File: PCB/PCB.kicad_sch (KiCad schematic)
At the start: 45 parts, among them J2 USB_C_Receptacle_USB2.0_16P, J4 Conn_01x15_Pin, J5 Conn_01x15_Pin, SW1 SW_Push, SW2 SW_Push, U2 ESP32-S3FN8, U3 TPS63900DSKR, Y1 40MHz

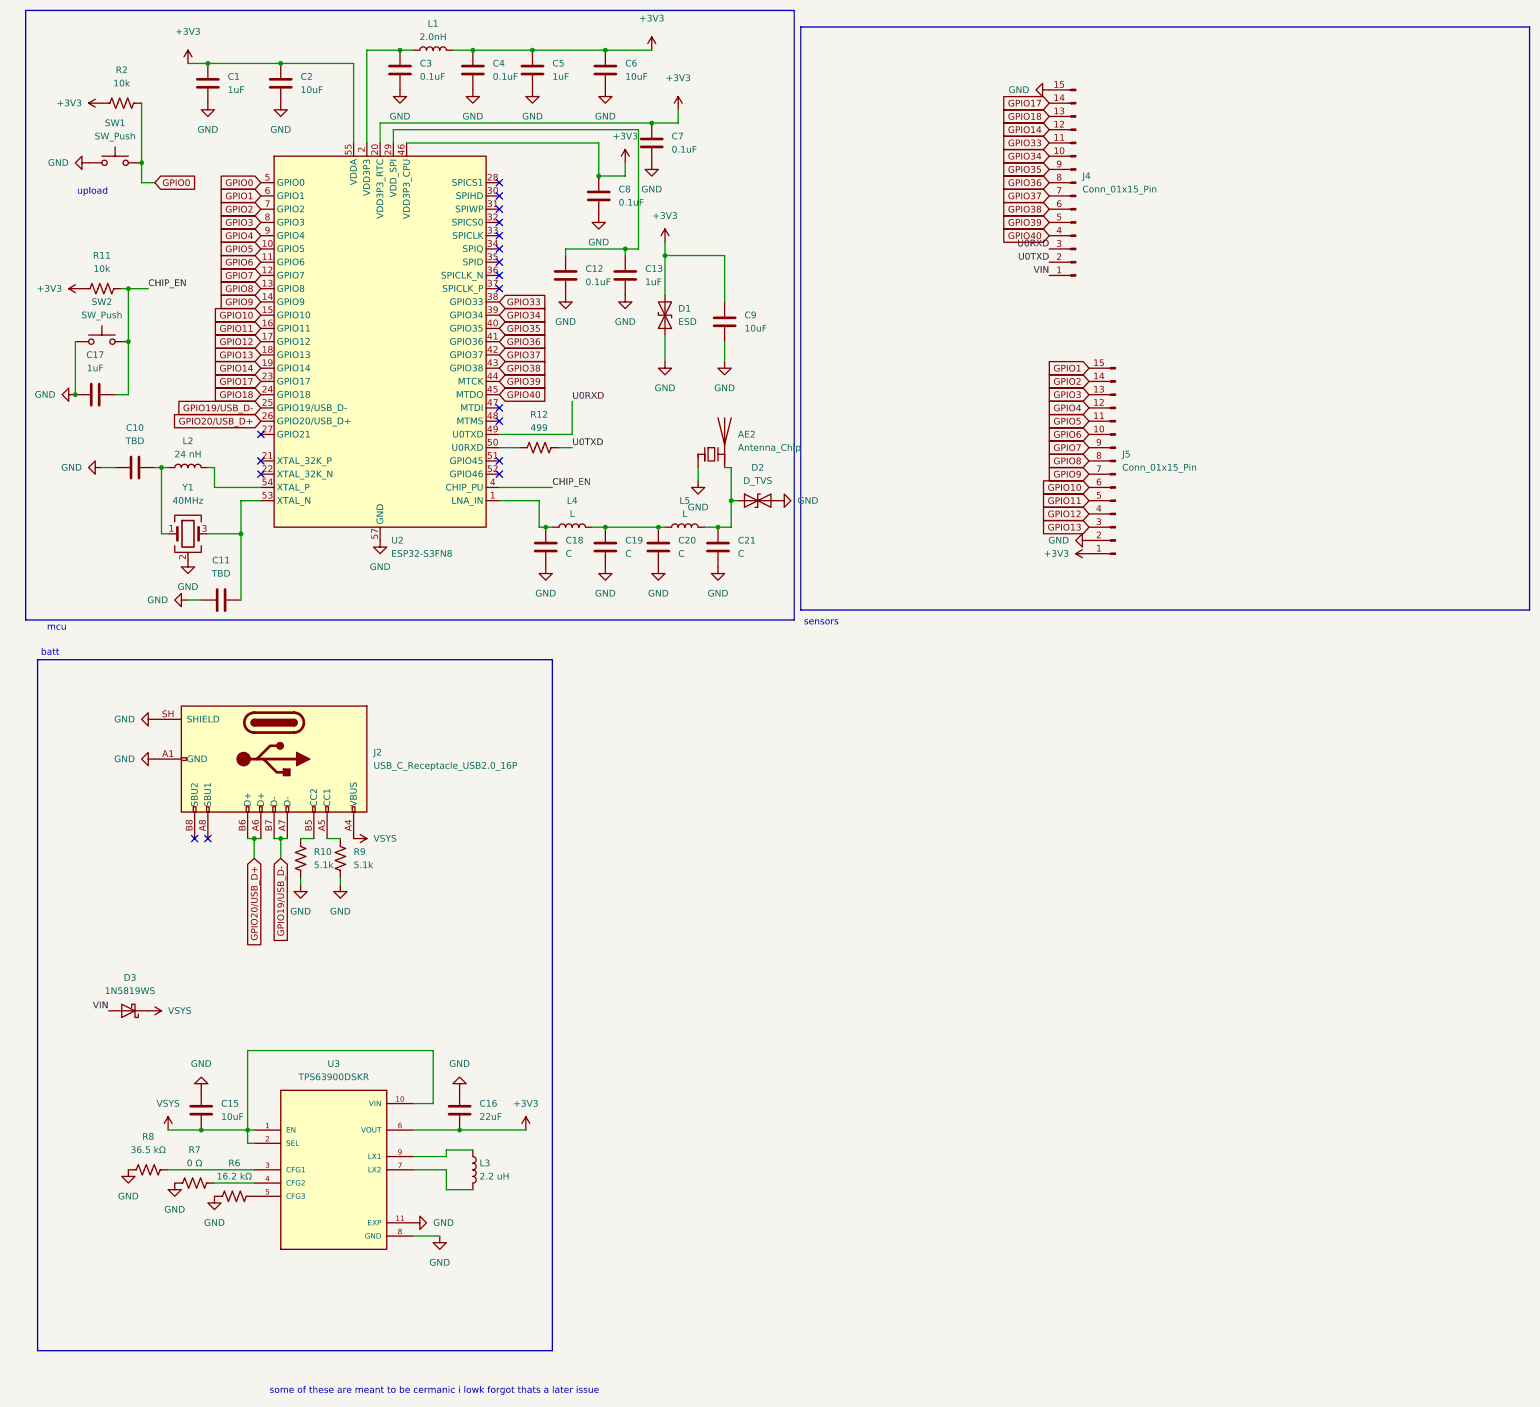
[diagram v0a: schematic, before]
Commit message: pcb work before big revision
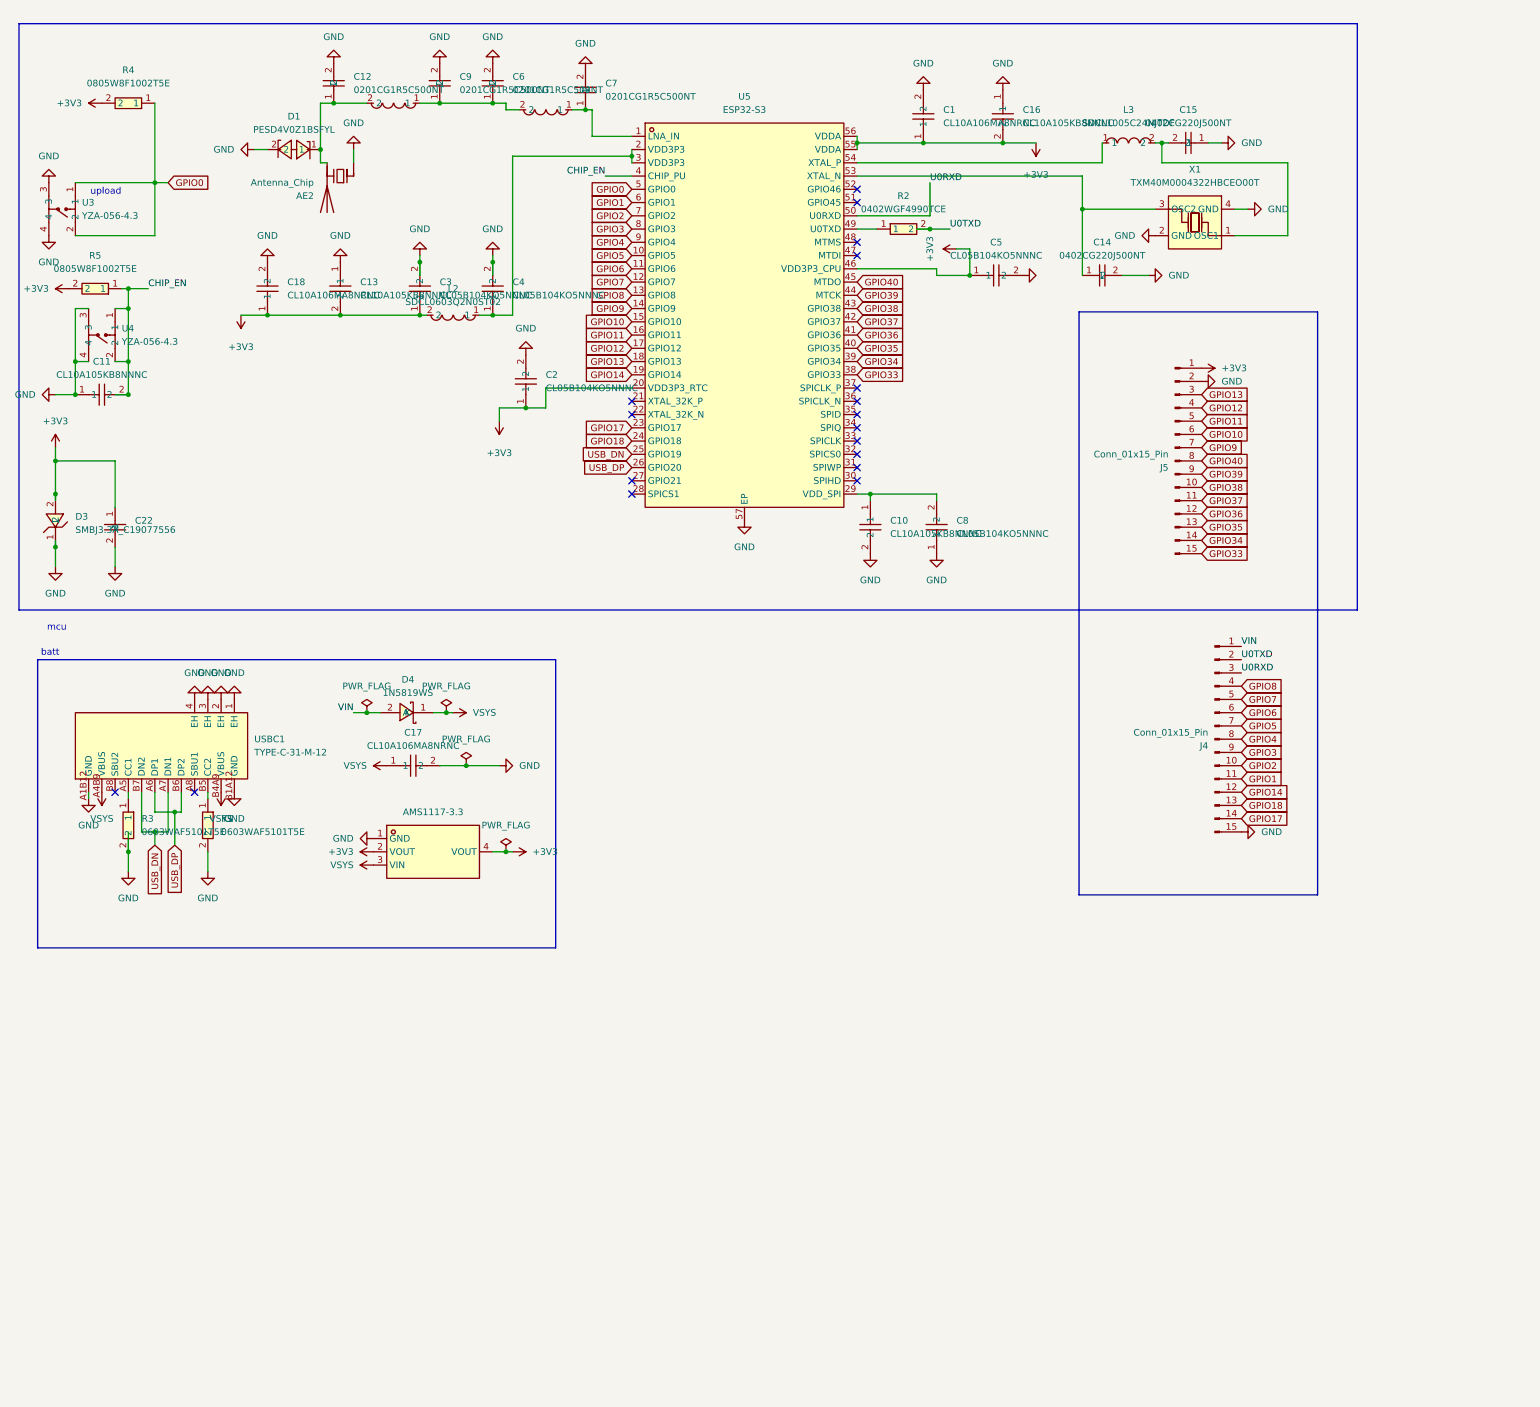
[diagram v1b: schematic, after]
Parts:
- removed C1, C13, C17, C5: 1uF, symbol Device:C
- removed C10, C11: TBD, symbol Device:C
- removed C12, C3, C4, C7, C8: 0.1uF, symbol Device:C
- removed C15, C2, C6, C9: 10uF, symbol Device:C
- removed C16: 22uF, symbol Device:C
- removed C18, C19, C20, C21: C, symbol Device:C
- removed D1: ESD, symbol Device:D_TVS
- removed D2: D_TVS, symbol Device:D_TVS
- removed D3: 1N5819WS, Diode_SMD:D_SOD-323, symbol Device:D_Schottky
- removed J2: USB_C_Receptacle_USB2.0_16P, symbol Connector:USB_C_Receptacle_USB2.0_16P
- removed L1: 2.0nH, symbol Device:L
- removed L2: 24 nH, symbol Device:L
- removed L3: 2.2 uH, symbol Device:L
- removed L4, L5: L, symbol Device:L
- removed R10, R9: 5.1k, symbol Device:R_US
- removed R11, R2: 10k, symbol Device:R_US
- removed R12: 499, symbol Device:R_US
- removed R6: 16.2 kΩ, symbol Device:R_US
- removed R7: 0 Ω, symbol Device:R_US
- removed R8: 36.5 kΩ, symbol Device:R_US
- removed SW1, SW2: SW_Push, symbol Switch:SW_Push
- removed U2: ESP32-S3FN8, Package_DFN_QFN:QFN-56-1EP_7x7mm_P0.4mm_EP4x4mm, symbol MCU_Espressif:ESP32-S3
- removed U3: TPS63900DSKR, IC_TPS63900DSKR:IC_TPS63900DSKR, symbol TPS63900DSKR:TPS63900DSKR
- removed Y1: 40MHz, symbol Device:Crystal_GND24
- added C1, C17, C18: CL10A106MA8NRNC, easyeda2kicad:C0603, symbol easyeda:CL10A106MA8NRNC
- added C10, C11, C13, C16: CL10A105KB8NNNC, easyeda2kicad:C0603, symbol easyeda:CL10A105KB8NNNC
- added C12, C6, C7, C9: 0201CG1R5C500NT, easyeda2kicad:C0201, symbol easyeda:0201CG1R5C500NT
- added C14, C15: 0402CG220J500NT, easyeda2kicad:C0402, symbol easyeda:0402CG220J500NT
- added C2, C3, C4, C5, C8: CL05B104KO5NNNC, easyeda2kicad:C0402, symbol easyeda:CL05B104KO5NNNC
- added C22: CL31A106KBHNNNE, easyeda2kicad:C1206, symbol easyeda:CL31A106KBHNNNE
- added D1: PESD4V0Z1BSFYL, easyeda2kicad:DSN0603-2_L0.7-W0.3-P0.40-BI, symbol easyeda:PESD4V0Z1BSFYL
- added D3: SMBJ3.3A_C19077556, easyeda2kicad:SMB_L4.6-W3.6-LS5.3-RD, symbol easyeda:SMBJ3.3A_C19077556
- added D4: 1N5819WS, easyeda2kicad:SOD-323_L1.8-W1.3-LS2.5-RD, symbol easyeda:1N5819WS
- added L1, L2, L4: SDCL0603Q2N0ST02, easyeda2kicad:L0201, symbol easyeda:SDCL0603Q2N0ST02
- added L3: SDCL1005C24NJTDF, easyeda2kicad:L0402-RD, symbol easyeda:SDCL1005C24NJTDF
- added R1, R3: 0603WAF5101T5E, easyeda2kicad:R0603, symbol easyeda:0603WAF5101T5E
- added R2: 0402WGF4990TCE, easyeda2kicad:R0402, symbol easyeda:0402WGF4990TCE
- added R4, R5: 0805W8F1002T5E, easyeda2kicad:R0805, symbol easyeda:0805W8F1002T5E
- added U1: AMS1117-3.3, easyeda2kicad:SOT-223-3_L6.5-W3.4-P2.30-LS7.0-BR, symbol easyeda:AMS1117-3.3
- added U3, U4: YZA-056-4.3, easyeda2kicad:SW-SMD_4P-L4.5-W4.5-P3.00-LS6.8, symbol easyeda:YZA-056-4.3
- added U5: ESP32-S3, easyeda2kicad:QFN-56_L7.0-W7.0-P0.40-TL-EP4.0, symbol easyeda:ESP32-S3
- added USBC1: TYPE-C-31-M-12, easyeda2kicad:USB-C_SMD-TYPE-C-31-M-12_1, symbol easyeda:TYPE-C-31-M-12
- added X1: TXM40M0004322HBCEO00T, easyeda2kicad:CRYSTAL-SMD_4P-L3.2-W2.5-BL-2, symbol easyeda:TXM40M0004322HBCEO00T
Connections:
- net +3V3: now also C1.1, C13.2, C16.2, C18.1, C2.1, C22.1, C3.1, C5.1, D3.2, L2.2, R4.2, R5.2, U1.2 (VOUT), U1.4 (VOUT), U5.20 (VDD3P3_RTC), U5.46 (VDD3P3_CPU), U5.55 (VDDA), U5.56 (VDDA)
- net CHIP_EN: now also C11.2, R5.1, U4.1, U4.2, U5.4 (CHIP_PU)
- net GND: now also C1.2, C10.2, C11.1, C12.2, C13.1, C14.2, C15.1, C16.1, C17.2, C18.2, C2.2, C22.2, C3.2, C4.2, C5.2, C6.2, C7.2, C8.1, C9.2, D1.2, D3.1, R1.2, R3.2, U1.1 (GND), U3.3, U3.4, U4.3, U4.4, U5.57 (EP), USBC1.1 (EH), USBC1.2 (EH), USBC1.3 (EH), USBC1.4 (EH), USBC1.A1B12 (GND), USBC1.B1A12 (GND), X1.2 (GND), X1.4 (GND)
- net GPIO0: now also R4.1, U3.1, U3.2, U5.5 (GPIO0)
- net GPIO1: now also J4.11 (Pin_11), U5.6 (GPIO1); no longer J5.15 (Pin_15)
- net GPIO10: now also U5.15 (GPIO10)
- net GPIO11: now also U5.16 (GPIO11)
- net GPIO12: now also U5.17 (GPIO12)
- net GPIO13: now also U5.18 (GPIO13)
- net GPIO14: now also U5.19 (GPIO14)
- net GPIO17: now also U5.23 (GPIO17)
- net GPIO18: now also U5.24 (GPIO18)
- net GPIO2: now also J4.10 (Pin_10), U5.7 (GPIO2); no longer J5.14 (Pin_14)
- net GPIO3: now also J4.9 (Pin_9), U5.8 (GPIO3); no longer J5.13 (Pin_13)
- net GPIO33: now also J5.15 (Pin_15), U5.38 (GPIO33); no longer J4.11 (Pin_11)
- net GPIO34: now also J5.14 (Pin_14), U5.39 (GPIO34); no longer J4.10 (Pin_10)
- net GPIO35: now also J5.13 (Pin_13), U5.40 (GPIO35); no longer J4.9 (Pin_9)
- net GPIO36: now also J5.12 (Pin_12), U5.41 (GPIO36); no longer J4.8 (Pin_8)
- net GPIO37: now also J5.11 (Pin_11), U5.42 (GPIO37); no longer J4.7 (Pin_7)
- net GPIO38: now also J5.10 (Pin_10), U5.43 (GPIO38); no longer J4.6 (Pin_6)
- net GPIO39: now also J5.9 (Pin_9), U5.44 (MTCK); no longer J4.5 (Pin_5)
- net GPIO4: now also J4.8 (Pin_8), U5.9 (GPIO4); no longer J5.12 (Pin_12)
- net GPIO40: now also J5.8 (Pin_8), U5.45 (MTDO); no longer J4.4 (Pin_4)
- net GPIO5: now also J4.7 (Pin_7), U5.10 (GPIO5); no longer J5.11 (Pin_11)
- net GPIO6: now also J4.6 (Pin_6), U5.11 (GPIO6); no longer J5.10 (Pin_10)
- net GPIO7: now also J4.5 (Pin_5), U5.12 (GPIO7); no longer J5.9 (Pin_9)
- net GPIO8: now also J4.4 (Pin_4), U5.13 (GPIO8); no longer J5.8 (Pin_8)
- net GPIO9: now also U5.14 (GPIO9)
- net U0RXD: now also U5.50 (U0RXD)
- net U0TXD: now also R2.2
- net VIN: now also D4.2 (A)
- net VSYS: now also C17.1, D4.1 (K), U1.3 (VIN), USBC1.A4B9 (VBUS), USBC1.B4A9 (VBUS)
- net at AE2.2 (PCB_Trace): now also C12.1, D1.1, L4.2
- new net: C6.1, C9.1, L1.2, L4.1
- new net: C7.1, L1.1, U5.1 (LNA_IN)
- new net: C15.2, L3.2, X1.1 (OSC1)
- new net: C14.1, U5.53 (XTAL_N), X1.3 (OSC2)
- new net: R3.1, USBC1.A5 (CC1)
- new net: C4.1, L2.1, U5.2 (VDD3P3), U5.3 (VDD3P3)
- new net: R1.1, USBC1.B5 (CC2)
- new net: L3.1, U5.54 (XTAL_P)
- new net: R2.1, U5.49 (U0TXD)
- new net: C10.1, C8.2, U5.29 (VDD_SPI)
- new net USB_DN: U5.25 (GPIO19), USBC1.A7 (DN1), USBC1.B7 (DN2)
- new net USB_DP: U5.26 (GPIO20), USBC1.A6 (DP1), USBC1.B6 (DP2)
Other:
- note removed: "sensors"
- note removed: "some of these are meant to be cermanic i lowk forgot thats a later issue"
- moved on the sheet: J4, J5
